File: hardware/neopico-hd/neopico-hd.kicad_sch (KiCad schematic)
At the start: 19 parts, among them J1 HDMI_A, U1 SN74LVC2G14DBV, U2 SN74LVC2G14DBV, U3 SN74LVC245APW, U4 SN74LVC245APW, U5 SN74LVC245APW, U6 ESD224DQA, U7 ESD224DQA

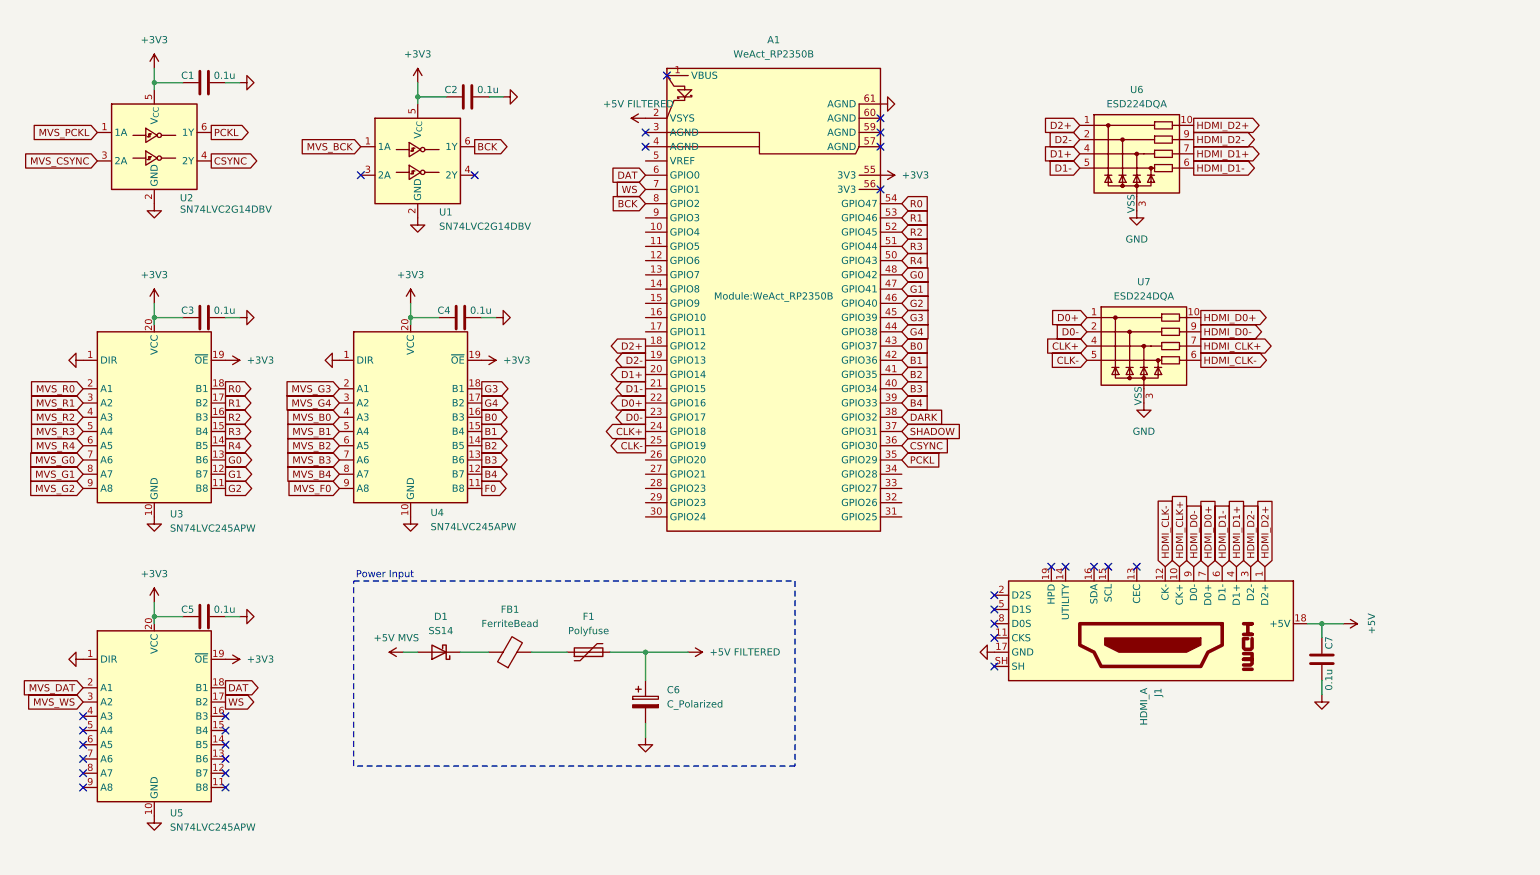
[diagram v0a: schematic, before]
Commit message: Starting PCB
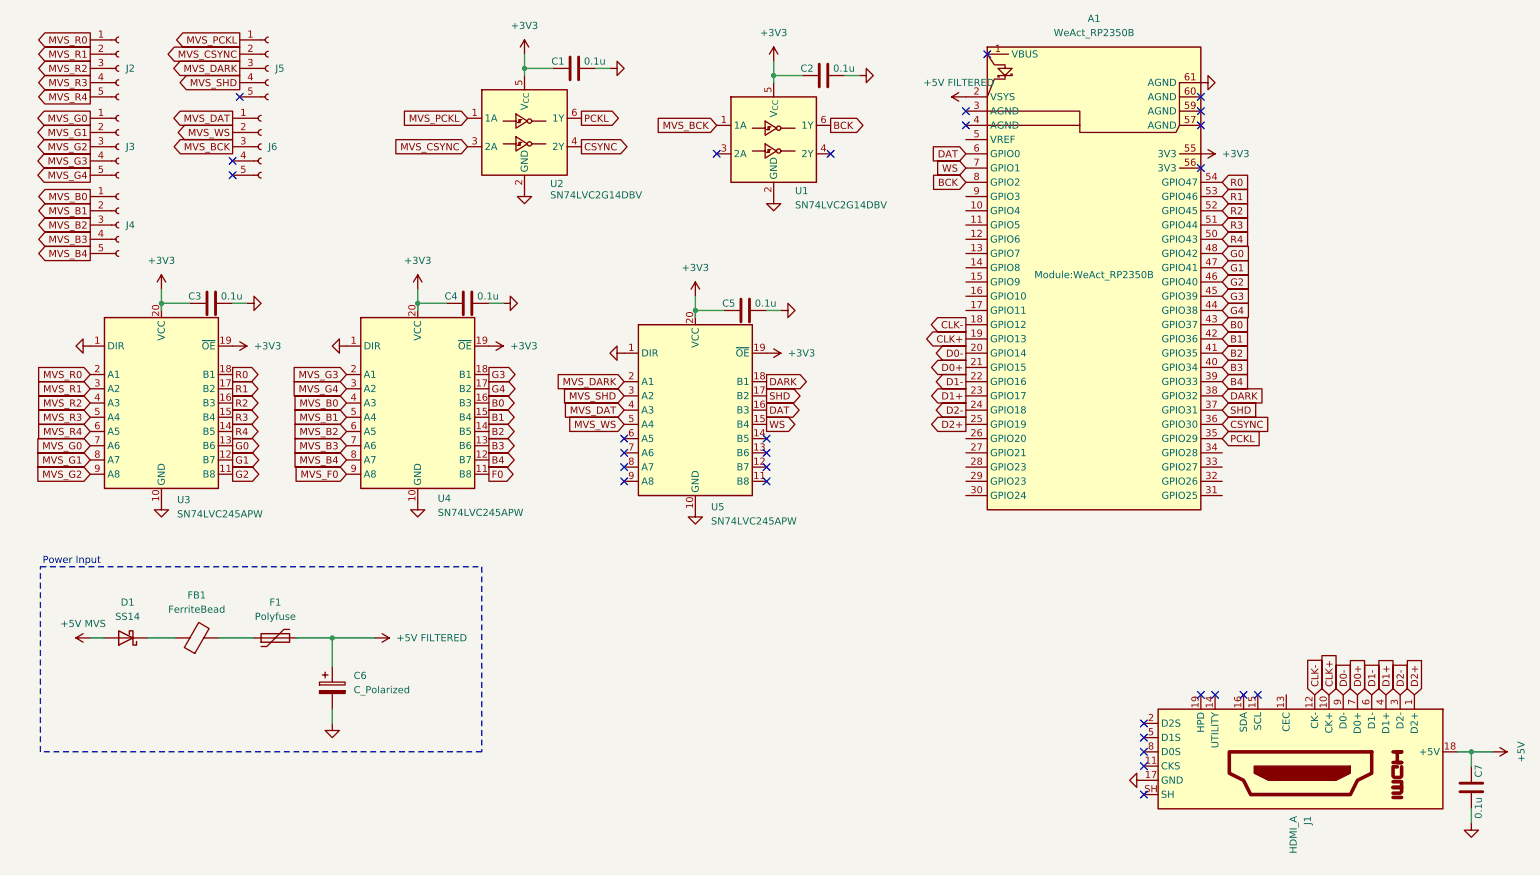
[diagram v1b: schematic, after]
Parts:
- removed U6, U7: ESD224DQA, Package_DFN_QFN:Diodes_UDFN-10_1.0x2.5mm_P0.5mm, symbol Power_Protection:ESD224DQA
- added J2, J3, J4: Conn_01x05_Socket, Connector_JST:JST_XH_B5B-XH-A_1x05_P2.50mm_Vertical, symbol Connector:Conn_01x05_Socket
- added J5, J6: Conn_01x05_Socket, symbol Connector:Conn_01x05_Socket
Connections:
- net HDMI_CLK+ is gone; now on net CLK+: J1.10 (CK+)
- net HDMI_CLK- is gone; now on net CLK-: J1.12 (CK-)
- net HDMI_D0+ is gone; now on net D0+: J1.7 (D0+)
- net HDMI_D0- is gone; now on net D0-: J1.9 (D0-)
- net HDMI_D1+ is gone; now on net D1+: J1.4 (D1+)
- net HDMI_D1- is gone; now on net D1-: J1.6 (D1-)
- net HDMI_D2+ is gone; now on net D2+: J1.1 (D2+)
- net HDMI_D2- is gone; now on net D2-: J1.3 (D2-)
- net CLK+: now also A1.19 (GPIO13); no longer A1.24 (GPIO18)
- net CLK-: now also A1.18 (GPIO12); no longer A1.25 (GPIO19)
- net D0+: now also A1.21 (GPIO15); no longer A1.22 (GPIO16)
- net D0-: now also A1.20 (GPIO14); no longer A1.23 (GPIO17)
- net D1+: now also A1.23 (GPIO17); no longer A1.20 (GPIO14)
- net D1-: now also A1.22 (GPIO16); no longer A1.21 (GPIO15)
- net D2+: now also A1.25 (GPIO19); no longer A1.18 (GPIO12)
- net D2-: now also A1.24 (GPIO18); no longer A1.19 (GPIO13)
- net DARK: now also U5.18 (B1)
- net DAT: now also U5.16 (B3); no longer U5.18 (B1)
- net MVS_B0: now also J4.1 (Pin_1)
- net MVS_B1: now also J4.2 (Pin_2)
- net MVS_B2: now also J4.3 (Pin_3)
- net MVS_B3: now also J4.4 (Pin_4)
- net MVS_B4: now also J4.5 (Pin_5)
- net MVS_BCK: now also J6.3 (Pin_3)
- net MVS_CSYNC: now also J5.2 (Pin_2)
- net MVS_DAT: now also U5.4 (A3), J6.1 (Pin_1); no longer U5.2 (A1)
- net MVS_G0: now also J3.1 (Pin_1)
- net MVS_G1: now also J3.2 (Pin_2)
- net MVS_G2: now also J3.3 (Pin_3)
- net MVS_G3: now also J3.4 (Pin_4)
- net MVS_G4: now also J3.5 (Pin_5)
- net MVS_PCKL: now also J5.1 (Pin_1)
- net MVS_R0: now also J2.1 (Pin_1)
- net MVS_R1: now also J2.2 (Pin_2)
- net MVS_R2: now also J2.3 (Pin_3)
- net MVS_R3: now also J2.4 (Pin_4)
- net MVS_R4: now also J2.5 (Pin_5)
- net MVS_WS: now also U5.5 (A4), J6.2 (Pin_2); no longer U5.3 (A2)
- net WS: now also U5.15 (B4); no longer U5.17 (B2)
- net SHADOW renamed SHD
- net SHD: now also U5.17 (B2)
- new net MVS_DARK: J5.3 (Pin_3), U5.2 (A1)
- new net MVS_SHD: J5.4 (Pin_4), U5.3 (A2)
- no-connect marks 31 -> 29
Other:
- moved on the sheet: A1, C1, C2, C3, C4, C5, C6, C7, D1, F1, FB1, J1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
